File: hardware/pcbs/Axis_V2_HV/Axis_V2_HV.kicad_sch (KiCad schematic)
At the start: 29 parts, among them J1 Screw_Terminal_01x03, J2 3WAY, J4 3WAY, J5 PUMP, K1 G2RL-1-E, Q1 BC847, Q2 BC847, U1 AQH3213, U2 AQH3213, U3 SZNUD3160

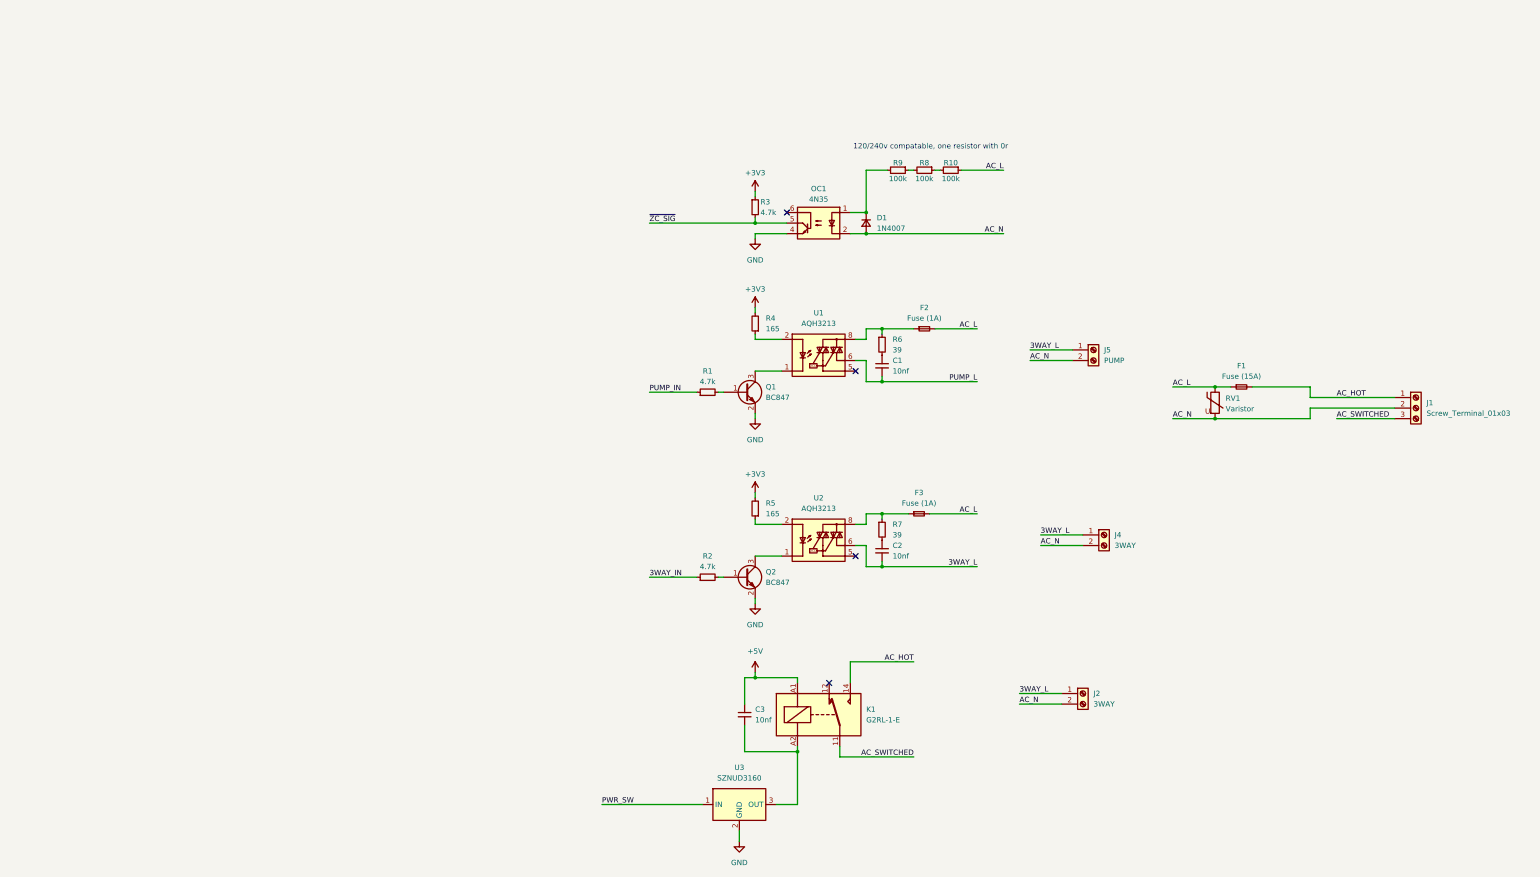
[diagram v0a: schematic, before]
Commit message: More updates and changes
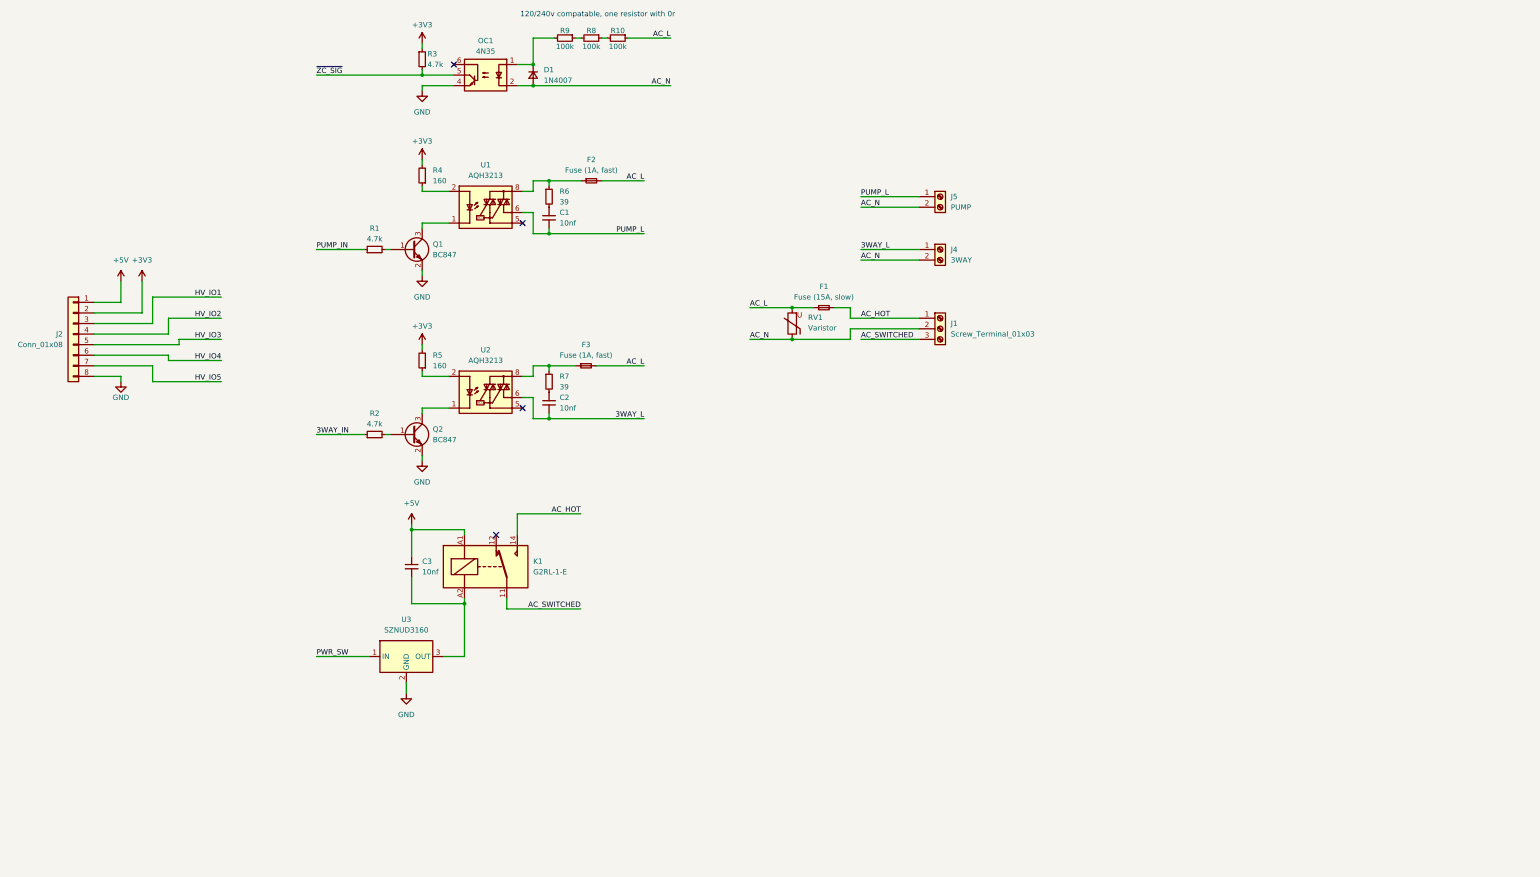
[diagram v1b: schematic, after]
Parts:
- removed J2: 3WAY, symbol Connector:Screw_Terminal_01x02
- added J2: Conn_01x08, Connector_IDC:IDC-Header_2x04_P2.54mm_Vertical, symbol Connector_Generic:Conn_01x08
- F1: value Fuse (15A) -> Fuse (15A, slow)
- F2, F3: value Fuse (1A) -> Fuse (1A, fast)
- R4, R5: value 165 -> 160
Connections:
- net +3V3: now also J2.2 (Pin_2)
- net +5V: now also J2.1 (Pin_1)
- net 3WAY_L: no longer J5.1 (Pin_1)
- net AC_L: now also RV1.2; no longer RV1.1
- net AC_N: now also RV1.1; no longer RV1.2
- net GND: now also J2.8 (Pin_8)
- net PUMP_L: now also J5.1 (Pin_1)
- new net HV_IO1: J2.3 (Pin_3)
- new net HV_IO2: J2.4 (Pin_4)
- new net HV_IO3: J2.5 (Pin_5)
- new net HV_IO4: J2.6 (Pin_6)
- new net HV_IO5: J2.7 (Pin_7)
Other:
- moved on the sheet: C1, C2, C3, D1, F1, F2, F3, J1, J4, J5, K1, OC1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
